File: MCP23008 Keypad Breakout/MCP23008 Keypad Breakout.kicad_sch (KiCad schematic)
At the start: 15 parts, among them J1 Conn_01x08_Pin, J2 RJ45_Shielded, U1 MCP23008-xP

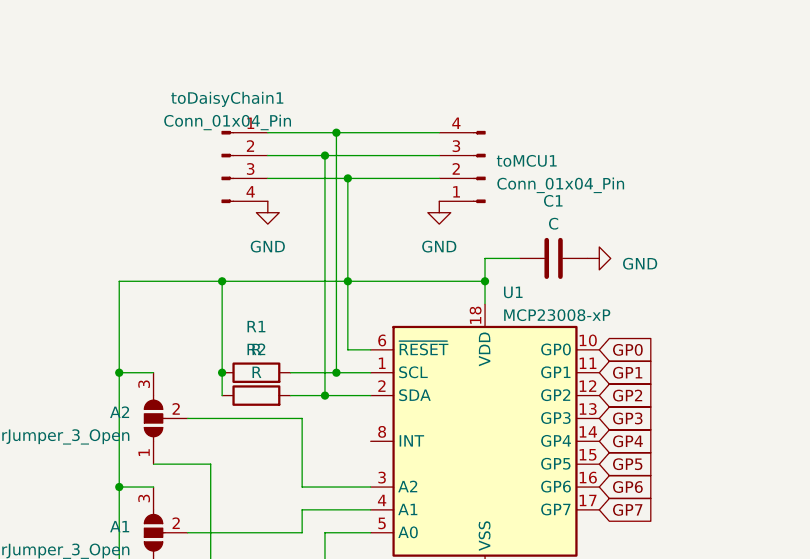
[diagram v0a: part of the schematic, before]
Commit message: asdf
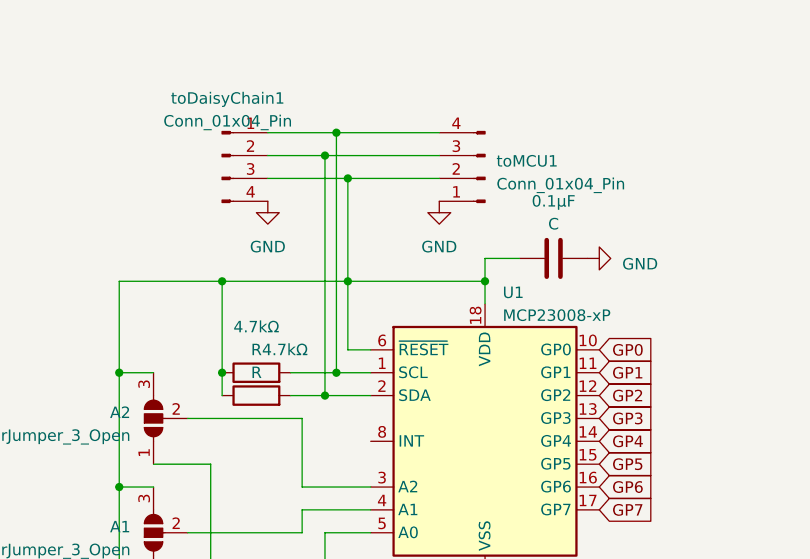
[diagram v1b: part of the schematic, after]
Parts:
- renumbered C1 to 0.1μF, R2 to 4.7kΩ, R1 to 4.7kΩ
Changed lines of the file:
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@@
   (symbol (lib_id "Device:C") (at 149.86 62.23 90) (unit 1)
     (in_bom yes) (on_board yes) (dnp no) (fields_autoplaced)
-    (property "Reference" "C1" (at 149.86 55.88 90)
+    (property "Reference" "0.1μF" (at 149.86 55.88 90)
       (effects (font (size 1.27 1.27)))
     )
@@
       (project "MCP23008 Keypad Breakout"
         (path "/06961e75-9629-4ee8-a7dc-c0a8ae24d9cc"
-          (reference "C1") (unit 1)
+          (reference "0.1μF") (unit 1)
         )
       )
@@
   )
   (symbol (lib_id "Device:R") (at 116.84 77.47 90) (unit 1)
-    (in_bom yes) (on_board yes) (dnp no) (fields_autoplaced)
-    (property "Reference" "R2" (at 116.84 72.39 90)
+    (in_bom yes) (on_board yes) (dnp no)
+    (property "Reference" "4.7kΩ" (at 120.015 72.39 90)
       (effects (font (size 1.27 1.27)))
     )
@@
       (project "MCP23008 Keypad Breakout"
         (path "/06961e75-9629-4ee8-a7dc-c0a8ae24d9cc"
-          (reference "R2") (unit 1)
+          (reference "4.7kΩ") (unit 1)
         )
       )
@@
   (symbol (lib_id "Device:R") (at 116.84 74.93 90) (unit 1)
     (in_bom yes) (on_board yes) (dnp no) (fields_autoplaced)
-    (property "Reference" "R1" (at 116.84 69.85 90)
+    (property "Reference" "4.7kΩ" (at 116.84 69.85 90)
       (effects (font (size 1.27 1.27)))
     )
@@
       (project "MCP23008 Keypad Breakout"
         (path "/06961e75-9629-4ee8-a7dc-c0a8ae24d9cc"
-          (reference "R1") (unit 1)
-        )
-      )
+          (reference "4.7kΩ") (unit 1)
+        )
+      )
